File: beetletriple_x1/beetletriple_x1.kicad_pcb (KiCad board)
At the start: 4 copper layers, 82 x 56.5 mm, 85 parts, among them J1 Power IN, J10 soicbite programming connector, J2 motor_out, J3 motor_out, J4 motor_out, J5 input_c1, J6 input_c2, J7 input_c3, J8 output_c4, J9 output_c5, Q1 IRF8313PBF, Q2 IRF8313PBF, Q3 IRF8313PBF, Q4 IRF8313PBF, Q5 IRF8313PBF, Q6 IRF8313PBF, U1 TPS54331DR, U11 NCP81155MNTXG, U12 NCP81155MNTXG, U2 HT7550-1, U3 ATtiny1617-M, U4 78L12G-AB3-R, U5 NCP81155MNTXG, U6 NCP81155MNTXG, U7 NCP81155MNTXG, U8 NCP81155MNTXG

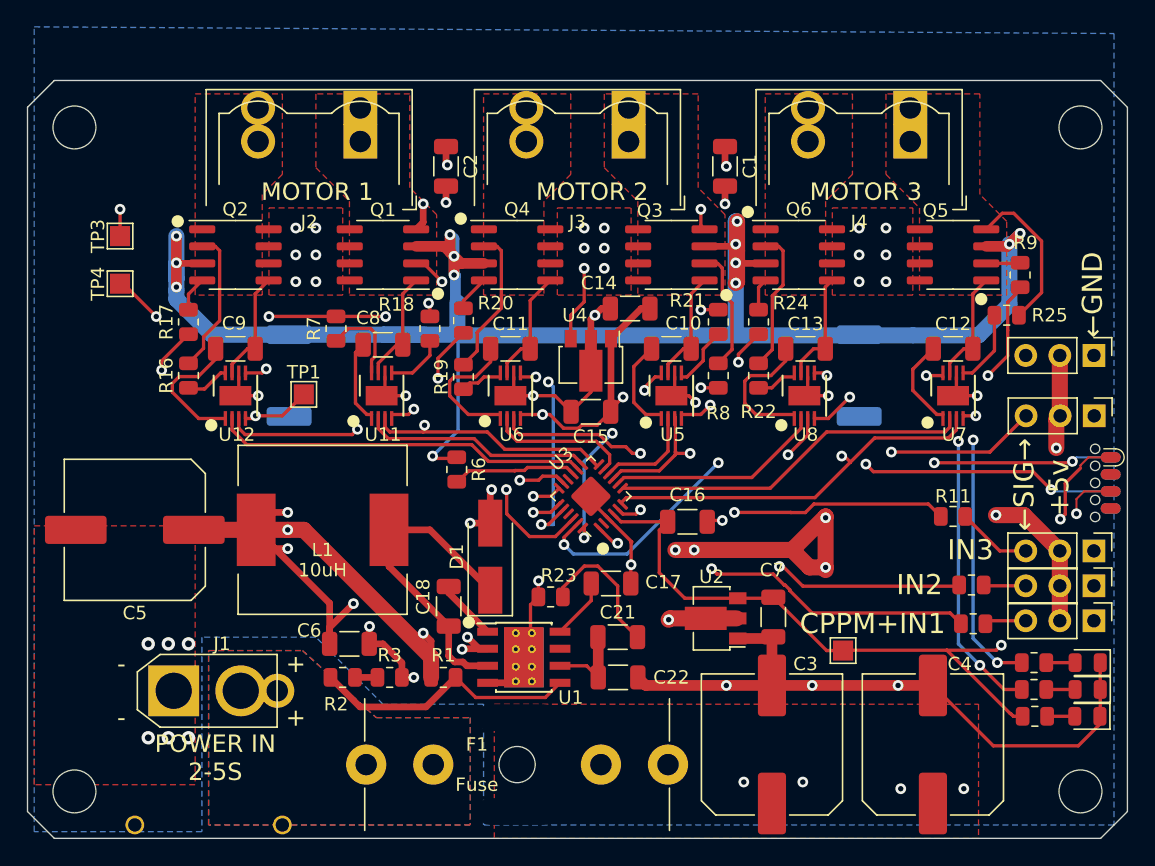
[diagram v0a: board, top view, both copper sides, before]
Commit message: minor updates
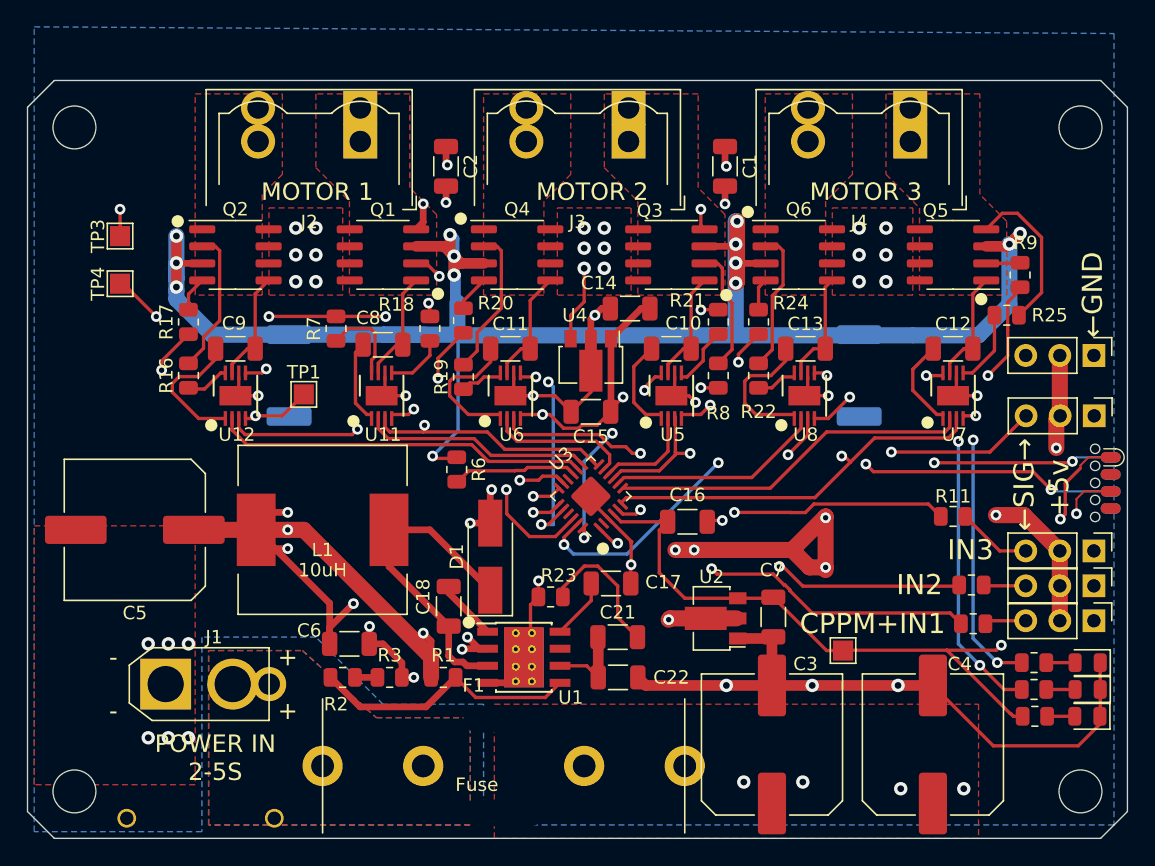
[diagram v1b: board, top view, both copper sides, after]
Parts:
- F1: footprint beetletriple:fuseholder_flexible -> beetletriple:fuseholder_bs1363
- moved F1 3.25 mm to (118.0, 131.6)
- moved J1 0.78 mm to (106.4, 125.5)
